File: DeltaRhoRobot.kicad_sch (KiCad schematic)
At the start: 31 parts, among them J1 Conn_01x02_Socket, J2 USB_C_Receptacle_USB2.0, J3 USB_C_Receptacle_USB2.0, Q3 STB55NF06T4, SW1 CAS-120A1, U1 AP63205WU-7, U2 AMS1117-3.3

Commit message: JLCniceness
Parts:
- J2, J3: JLCPCB Position Offset 0.91,0 -> 0,-0.91
- Q3: JLCPCB Position Offset 1.4,0 -> 0,1.4
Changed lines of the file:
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@@
 			)
 		)
-		(property "JLCPCB Position Offset" "0.91,0"
+		(property "JLCPCB Position Offset" "0,-0.91"
 			(at 32.766 42.418 0)
 			(effects
@@
 			)
 		)
-		(property "JLCPCB Position Offset" "0.91,0"
+		(property "JLCPCB Position Offset" "0,-0.91"
 			(at 31.496 110.363 0)
 			(effects
@@
 			)
 		)
-		(property "JLCPCB Position Offset" "1.4,0"
+		(property "JLCPCB Position Offset" "0,1.4"
 			(at 111.506 63.373 0)
 			(effects

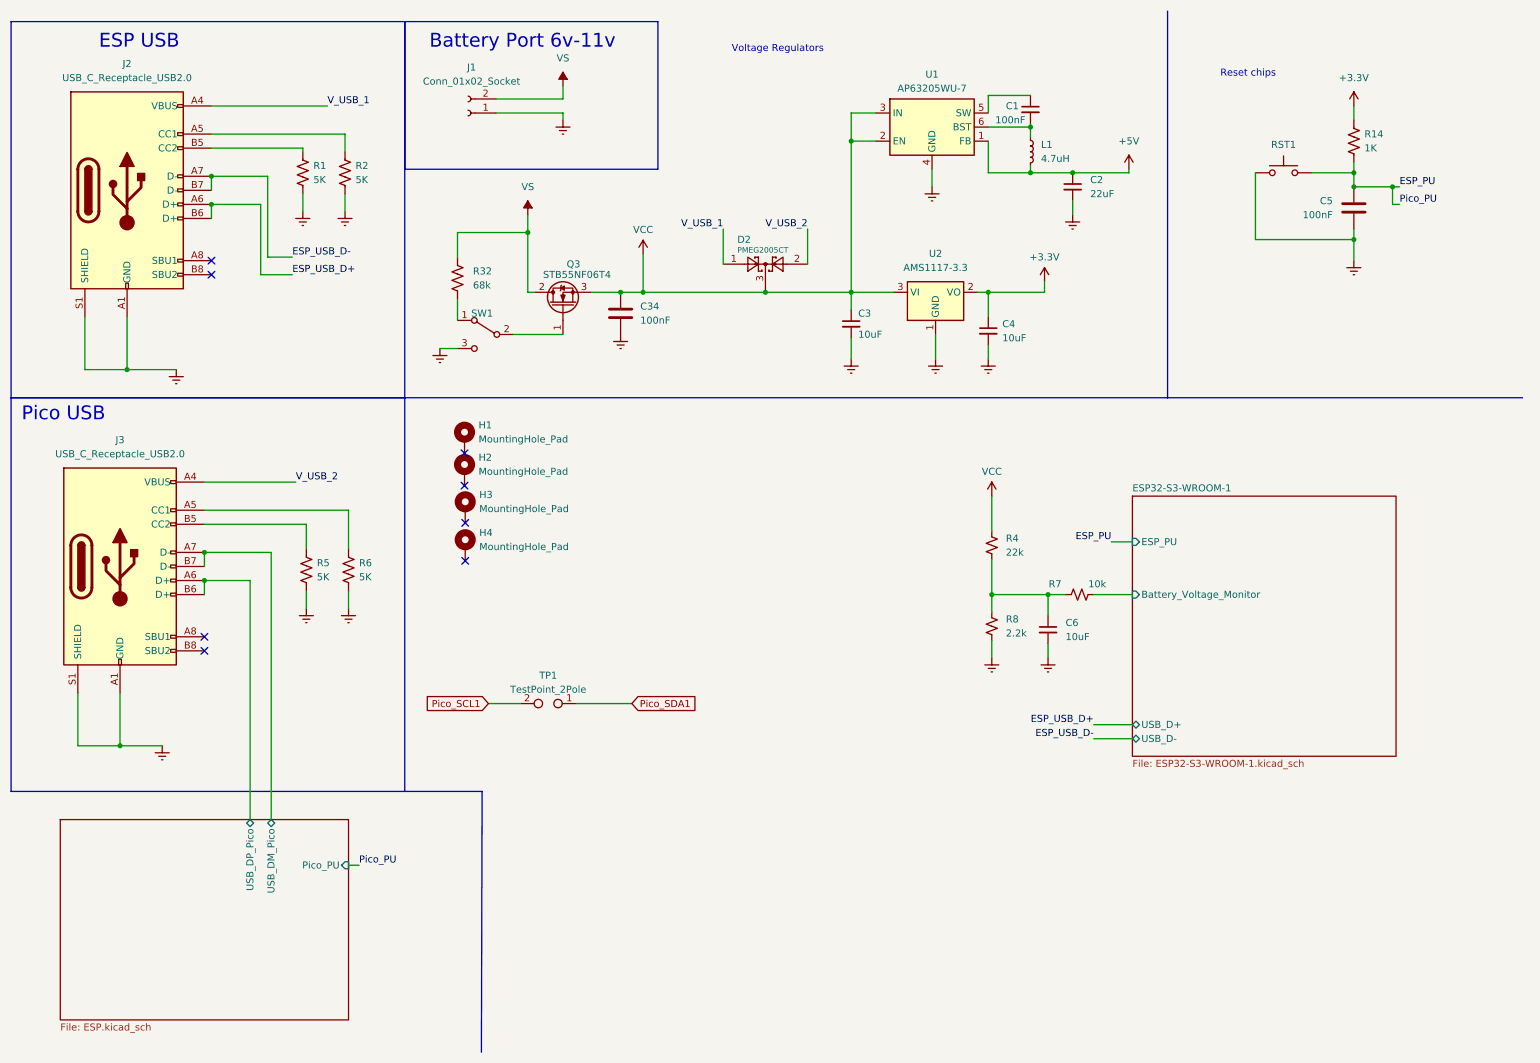
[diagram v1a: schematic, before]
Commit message: Rev 2 PCB
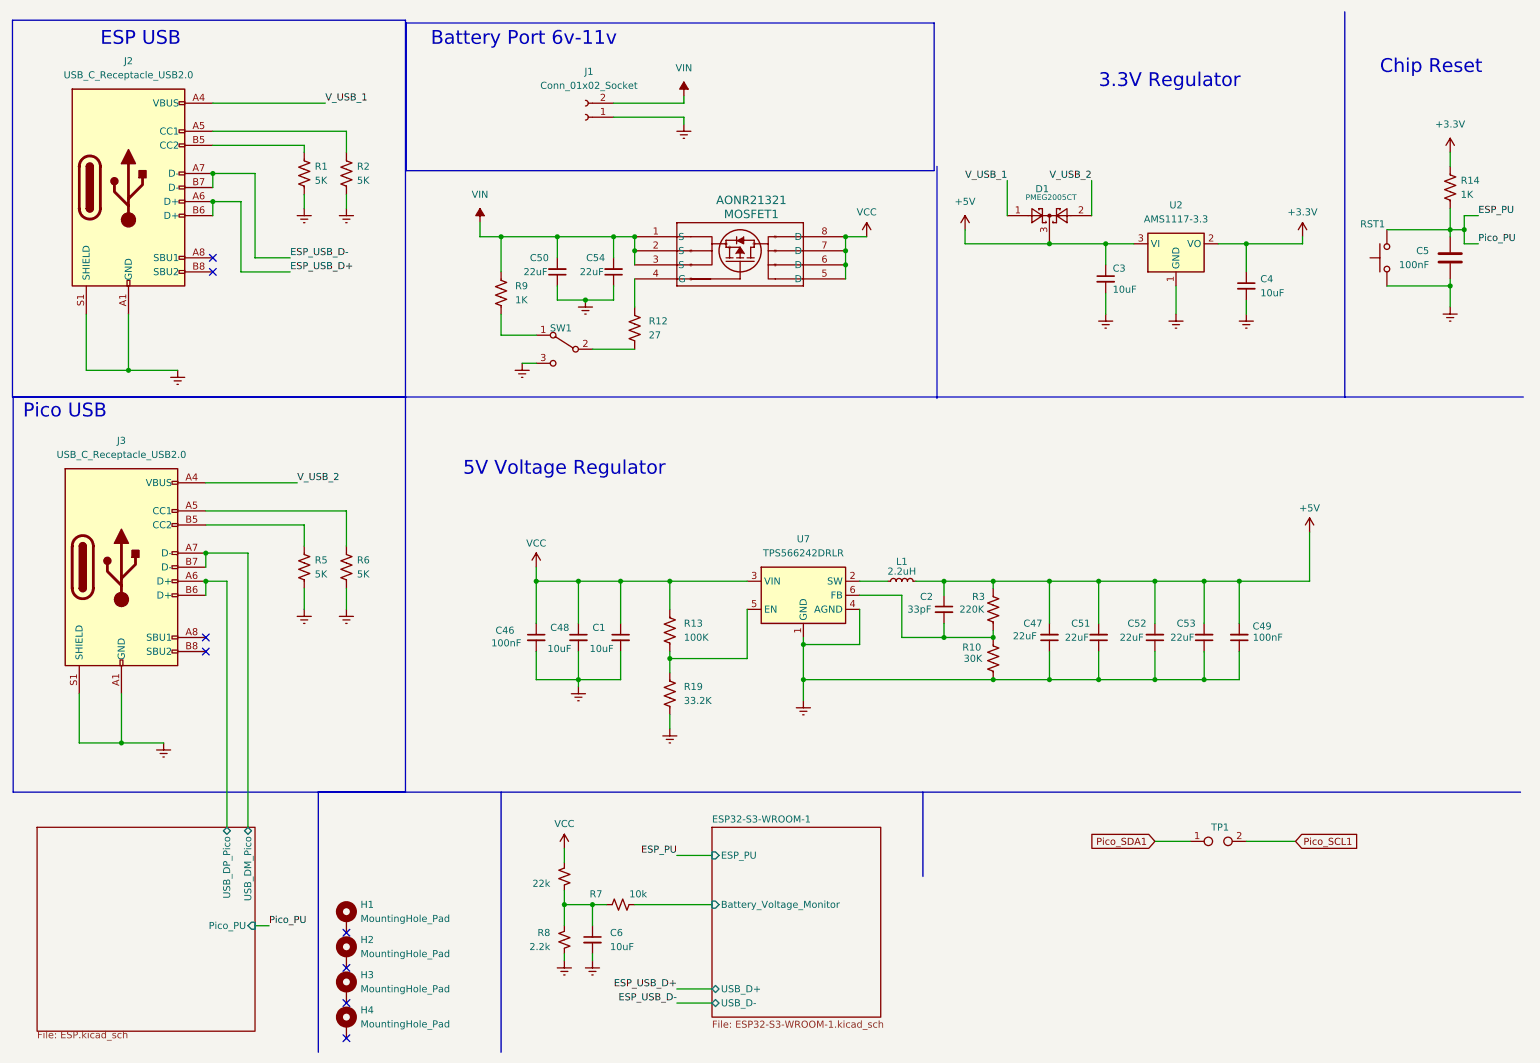
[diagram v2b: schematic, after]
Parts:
- removed C34: 100nF, Capacitor_SMD:C_0402_1005Metric, symbol Device:C
- removed D2: PMEG2005CT, Package_TO_SOT_SMD:SOT-23, symbol Diode:BAT54C
- removed Q3: STB55NF06T4, Package_TO_SOT_SMD:TO-263-2, symbol Device:Q_NMOS_Depletion_GDS
- removed R32: 68k, Resistor_SMD:R_0805_2012Metric, symbol Device:R_US
- removed U1: AP63205WU-7, Package_TO_SOT_SMD:TSOT-23-6, symbol Regulator_Switching:AP63205WU
- added C46, C49: 100nF, Capacitor_SMD:C_0402_1005Metric, symbol Device:C_Small
- added C47, C50, C51, C52, C53, C54: 22uF, Capacitor_SMD:C_0805_2012Metric, symbol Device:C_Small
- added C48: 10uF, Capacitor_SMD:C_0402_1005Metric, symbol Device:C_Small
- added D1: PMEG2005CT, Package_TO_SOT_SMD:SOT-23, symbol Diode:BAT54C
- added MOSFET1: AONR21321, AONR:DFN8_3x3_EP_AOS, symbol AONR21321:AONR21321
- added R10: 30K, Resistor_SMD:R_0402_1005Metric, symbol Device:R_US
- added R12: 27, Resistor_SMD:R_0402_1005Metric, symbol Device:R_US
- added R13: 100K, Resistor_SMD:R_0402_1005Metric, symbol Device:R_US
- added R19: 33.2K, Resistor_SMD:R_0402_1005Metric, symbol Device:R_US
- added R3: 220K, Resistor_SMD:R_0402_1005Metric, symbol Device:R_US
- added R9: 1K, Resistor_SMD:R_0402_1005Metric, symbol Device:R_US
- added U7: TPS566242DRLR, Package_TO_SOT_SMD:SOT-23-6, symbol Regulator_Switching:TPS565208
- C1: value 100nF -> 10uF
- C2: value 22uF -> 33pF; footprint Capacitor_SMD:C_Elec_6.3x5.8 -> Capacitor_SMD:C_0402_1005Metric; LCSC Part # C445459 -> C1525
- C3: footprint Capacitor_SMD:C_0805_2012Metric -> Capacitor_SMD:C_0402_1005Metric
- L1: value 4.7uH -> 2.2uH
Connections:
- net +5V: now also C3.1, U2.3 (VI), C47.2, C49.2, C51.2, C52.2, C53.2, D1.3, R3.1
- net Earth: now also C1.2, C46.2, C47.1, C48.2, C49.1, C50.1, C51.1, C52.1, C53.1, C54.1, R10.2, R19.2, U7.1 (GND), U7.4 (AGND); no longer C2.2
- net VCC: now also C1.1, C46.1, C48.1, MOSFET1.5 (D), MOSFET1.6 (D), MOSFET1.7 (D), MOSFET1.8 (D), R13.1, U7.3 (VIN); no longer C3.1, U2.3 (VI)
- net V_USB_1: now also D1.1
- net V_USB_2: now also D1.2
- net at SW1.1 (A): now also R9.2
- net at SW1.2 (B): now also R12.2
- net at L1.1: now also U7.2 (SW); no longer C1.2
- net VS renamed VIN
- net VIN: now also C50.2, C54.2, MOSFET1.1 (S), MOSFET1.2 (S), MOSFET1.3 (S), R9.1
- new net: R13.2, R19.1, U7.5 (EN)
- new net: MOSFET1.4 (G), R12.1
- new net: C2.2, R10.1, R3.2, U7.6 (FB)
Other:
- note added: "3.3V Regulator"
- note added: "5V Voltage Regulator"
- note added: "Chip Reset"
- note removed: "Reset chips"
- note removed: "Voltage Regulators"
- moved on the sheet: C5, C6, H1, H2, H3, H4, J1, J2, R14, R5, R6, R7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

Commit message: Rev 2 finished
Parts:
- C2: LCSC Part # C1525 -> C1562
- C3: footprint Capacitor_SMD:C_0402_1005Metric -> Capacitor_SMD:C_1206_3216Metric; LCSC Part # C15850 -> C13585
- C4: footprint Capacitor_SMD:C_0402_1005Metric -> Capacitor_SMD:C_1206_3216Metric; LCSC Part # C15525 -> C13585
- C46, C49, C5: LCSC Part # C1525 -> C307331
- C47, C50, C51, C52, C53, C54: LCSC Part # C445459 -> C45783
- C6: LCSC Part # C15525 -> C15525
- MOSFET1: LCSC Part # (none) -> C541711
- R10: footprint Resistor_SMD:R_0402_1005Metric -> Resistor_SMD:R_0603_1608Metric; LCSC Part # C25905 -> C22984
- R12: LCSC Part # C25905 -> C25105
- R13: LCSC Part # C25905 -> C25741
- R19: LCSC Part # C25905 -> C25779
- R3: footprint Resistor_SMD:R_0402_1005Metric -> Resistor_SMD:R_0603_1608Metric; LCSC Part # C25905 -> (none)
- R9: LCSC Part # C25905 -> C11702
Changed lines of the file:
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@@
 			)
 		)
-		(property "LCSC Part #" "C25905"
+		(property "LCSC Part #" "C25779"
 			(at 130.81 133.35 0)
 			(effects
@@
 			)
 		)
-		(property "LCSC Part #" "C15525"
+		(property "LCSC Part #" "C15525 "
 			(at 116.84 177.8 0)
 			(effects
@@
 			)
 		)
+		(property "LCSC Part #" "C541711"
+			(at 121.92 50.8 0)
+			(effects
+				(font
+					(size 1.27 1.27)
+				)
+				(hide yes)
+			)
+		)
 		(pin "1"
 		)
@@
 			)
 		)
-		(property "Footprint" "Capacitor_SMD:C_0402_1005Metric"
+		(property "Footprint" "Capacitor_SMD:C_1206_3216Metric"
 			(at 209.55 58.42 0)
 			(effects
@@
 			)
 		)
-		(property "LCSC Part #" "C15850"
+		(property "LCSC Part #" "C13585"
 			(at 209.55 58.42 0)
 			(effects
@@
 			)
 		)
-		(property "LCSC Part #" "C1525"
+		(property "LCSC Part #" "C1562"
 			(at 180.34 118.11 0)
 			(effects
@@
 			)
 		)
-		(property "LCSC Part #" "C1525"
+		(property "LCSC Part #" "C307331"
 			(at 271.78 54.61 0)
 			(effects
@@
 			)
 		)
-		(property "LCSC Part #" "C445459"
+		(property "LCSC Part #" "C45783"
 			(at 208.28 123.19 0)
 			(effects
@@
 			)
 		)
-		(property "LCSC Part #" "C1525"
+		(property "LCSC Part #" "C307331"
 			(at 233.68 123.19 0)
 			(effects
@@
 			)
 		)
-		(property "LCSC Part #" "C25905"
+		(property "LCSC Part #" "C25105"
 			(at 124.46 67.31 0)
 			(effects
@@
 			)
 		)
-		(property "LCSC Part #" "C25905"
+		(property "LCSC Part #" "C25741"
 			(at 130.81 121.92 0)
 			(effects
@@
 			)
 		)
-		(property "Footprint" "Resistor_SMD:R_0402_1005Metric"
+		(property "Footprint" "Resistor_SMD:R_0603_1608Metric"
 			(at 190.246 127.254 90)
 			(effects
@@
 			)
 		)
-		(property "LCSC Part #" "C25905"
+		(property "LCSC Part #" "C22984"
 			(at 189.23 127 0)
 			(effects
@@
 			)
 		)
-		(property "Footprint" "Capacitor_SMD:C_0402_1005Metric"
+		(property "Footprint" "Capacitor_SMD:C_1206_3216Metric"
 			(at 234.95 59.69 0)
 			(effects
@@
 			)
 		)
-		(property "LCSC Part #" "C15525"
+		(property "LCSC Part #" "C13585"
 			(at 234.95 59.69 0)
 			(effects
@@
 			)
 		)
-		(property "LCSC Part #" "C25905"
+		(property "LCSC Part #" "C11702"
 			(at 100.33 60.96 0)
 			(effects
@@
 			)
 		)
-		(property "LCSC Part #" "C445459"
+		(property "LCSC Part #" "C45783"
 			(at 227.33 123.19 0)
 			(effects
@@
 			)
 		)
-		(property "LCSC Part #" "C445459"
+		(property "LCSC Part #" "C45783"
 			(at 218.44 123.19 0)
 			(effects
@@
 			)
 		)
-		(property "LCSC Part #" "C1525"
+		(property "LCSC Part #" "C307331"
 			(at 106.68 123.19 0)
 			(effects
@@
 			)
 		)
-		(property "LCSC Part #" "C445459"
+		(property "LCSC Part #" "C45783"
 			(at 199.39 123.19 0)
 			(effects
@@
 			)
 		)
-		(property "LCSC Part #" "C445459"
+		(property "LCSC Part #" "C45783"
 			(at 110.49 57.15 0)
 			(effects
@@
 			)
 		)
-		(property "LCSC Part #" "C445459"
+		(property "LCSC Part #" "C45783"
 			(at 120.65 57.15 0)
 			(effects
@@
 			)
 		)
-		(property "Footprint" "Resistor_SMD:R_0402_1005Metric"
+		(property "Footprint" "Resistor_SMD:R_0603_1608Metric"
 			(at 190.246 118.364 90)
 			(effects
@@
 			)
 		)
-		(property "LCSC Part #" "C25905"
+		(property "LCSC Part #" ""
 			(at 189.23 118.11 0)
 			(effects

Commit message: Rev 3: fixing I2C and footprints
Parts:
- U7: footprint Package_TO_SOT_SMD:SOT-23-6 -> Package_TO_SOT_SMD:SOT-563
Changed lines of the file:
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@@
 			)
 		)
-		(property "Footprint" "Package_TO_SOT_SMD:SOT-23-6"
+		(property "Footprint" "Package_TO_SOT_SMD:SOT-563"
 			(at 156.21 121.92 0)
 			(effects
